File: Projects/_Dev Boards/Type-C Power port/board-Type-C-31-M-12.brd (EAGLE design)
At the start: 18.5 x 23 mm, 4 parts, among them J1 USB-TYPE-C-31-M-12

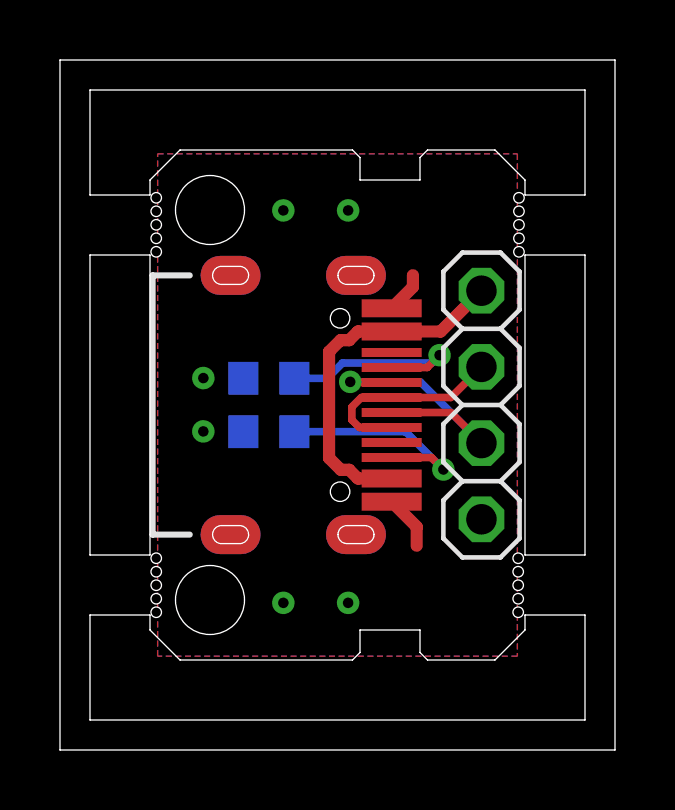
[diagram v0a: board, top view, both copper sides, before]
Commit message: update
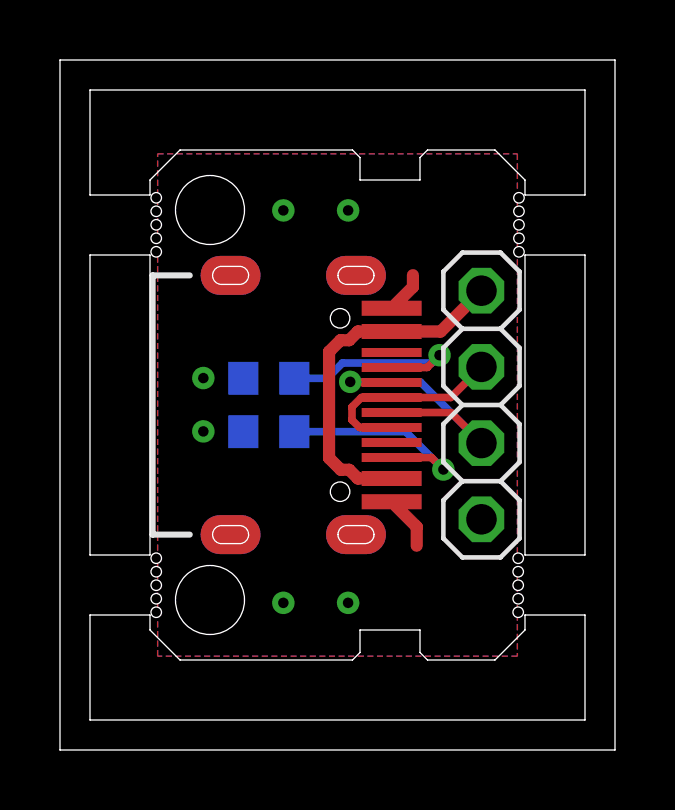
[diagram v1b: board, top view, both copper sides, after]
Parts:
- J1: device angrypig7-Connectors:USB-TYPE-C-31-M-12 -> angrypig7-Connectors-USB:USB-TYPE-C-31-M-12
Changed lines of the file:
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@@
 <setting verticaltext="up"/>
 </settings>
-<grid distance="5" unitdist="mil" unit="mil" style="lines" multiple="1" display="yes" altdistance="5" altunitdist="mil" altunit="mil"/>
+<grid distance="10" unitdist="mil" unit="mil" style="lines" multiple="1" display="yes" altdistance="5" altunitdist="mil" altunit="mil"/>
 <layers>
 <layer number="1" name="Top" color="4" fill="1" visible="yes" active="yes"/>
@@
 </autorouter>
 <elements>
-<element name="J1" library="angrypig7-Connectors" package="USB-TYPE-C-31-M-12" package3d_urn="urn:adsk.eagle:package:24334474/2" value="USB-TYPE-C-31-M-12" x="6.866" y="8.5" smashed="yes" rot="R270"/>
+<element name="J1" library="angrypig7-Connectors-USB" package="USB-TYPE-C-31-M-12" package3d_urn="urn:adsk.eagle:package:24334474/2" value="USB-TYPE-C-31-M-12" x="6.866" y="8.5" smashed="yes" rot="R270"/>
 <element name="R1" library="angrypig7-RCL" package="R0603" package3d_urn="urn:adsk.eagle:package:23555/54" value="5.1k" x="3.962" y="9.389" smashed="yes" rot="MR0">
 <attribute name="NAME" x="3.962" y="10.659" size="1.27" layer="28" font="vector" ratio="15" rot="MR0" align="center"/>
